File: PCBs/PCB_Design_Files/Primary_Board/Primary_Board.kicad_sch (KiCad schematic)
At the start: 6 parts, among them J1 Conn_FFC_8pin, J2 Conn_01x08_Pin

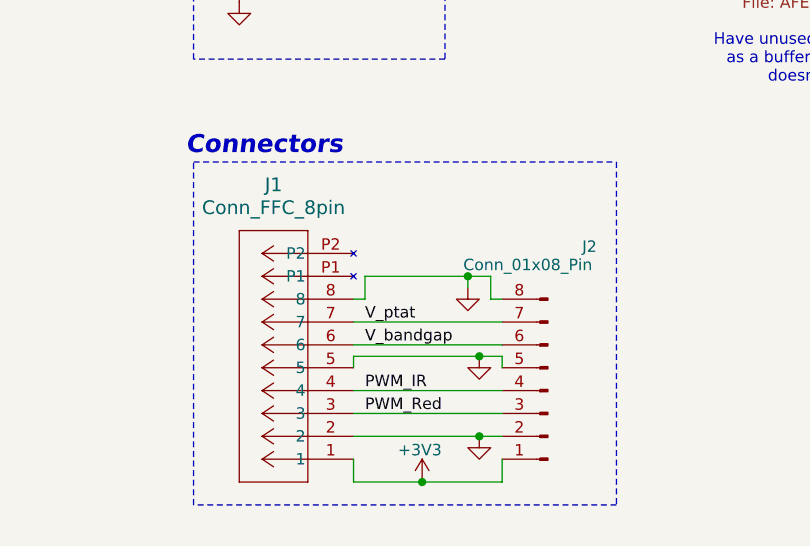
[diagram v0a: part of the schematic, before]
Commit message: updated bom
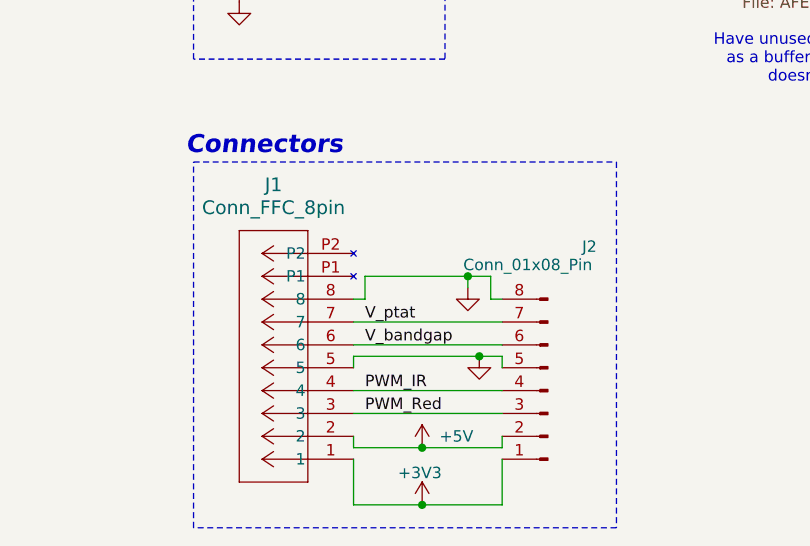
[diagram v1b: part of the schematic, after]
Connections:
- net GND: no longer J1.2, J2.2 (Pin_2)
- new net +5V: J1.2, J2.2 (Pin_2)
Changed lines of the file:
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@@
 	(rectangle
 		(start 25.4 93.98)
-		(end 72.39 132.08)
+		(end 72.39 134.62)
 		(stroke
 			(width 0)
@@
 	)
 	(junction
-		(at 50.8 129.54)
-		(diameter 0)
-		(color 0 0 0 0)
-	)
-	(junction
-		(at 57.15 124.46)
+		(at 50.8 132.08)
 		(diameter 0)
 		(color 0 0 0 0)
@@
 		(color 0 0 0 0)
 	)
+	(junction
+		(at 50.8 125.73)
+		(diameter 0)
+		(color 0 0 0 0)
+	)
 	(wire
 		(pts
@@
 	(wire
 		(pts
+			(xy 59.69 125.73) (xy 59.69 124.46)
+		)
+		(stroke
+			(width 0)
+			(type default)
+		)
+	)
+	(wire
+		(pts
 			(xy 58.42 106.68) (xy 58.42 109.22)
 		)
@@
 	(wire
 		(pts
-			(xy 57.15 124.46) (xy 59.69 124.46)
-		)
-		(stroke
-			(width 0)
-			(type default)
-		)
-	)
-	(wire
-		(pts
 			(xy 43.18 114.3) (xy 59.69 114.3)
 		)
@@
 	(wire
 		(pts
-			(xy 59.69 129.54) (xy 50.8 129.54)
+			(xy 59.69 132.08) (xy 50.8 132.08)
 		)
 		(stroke
@@
 	(wire
 		(pts
+			(xy 43.18 125.73) (xy 43.18 124.46)
+		)
+		(stroke
+			(width 0)
+			(type default)
+		)
+	)
+	(wire
+		(pts
 			(xy 44.45 106.68) (xy 55.88 106.68)
 		)
@@
 	(wire
 		(pts
-			(xy 43.18 127) (xy 43.18 129.54)
+			(xy 43.18 127) (xy 43.18 132.08)
 		)
 		(stroke
@@
 	(wire
 		(pts
-			(xy 43.18 124.46) (xy 57.15 124.46)
+			(xy 43.18 125.73) (xy 50.8 125.73)
 		)
 		(stroke
@@
 	(wire
 		(pts
+			(xy 50.8 125.73) (xy 59.69 125.73)
+		)
+		(stroke
+			(width 0)
+			(type default)
+		)
+	)
+	(wire
+		(pts
 			(xy 43.18 121.92) (xy 59.69 121.92)
 		)
@@
 	(wire
 		(pts
-			(xy 59.69 127) (xy 59.69 129.54)
-		)
-		(stroke
-			(width 0)
-			(type default)
-		)
-	)
-	(wire
-		(pts
-			(xy 43.18 129.54) (xy 50.8 129.54)
+			(xy 59.69 127) (xy 59.69 132.08)
+		)
+		(stroke
+			(width 0)
+			(type default)
+		)
+	)
+	(wire
+		(pts
+			(xy 43.18 132.08) (xy 50.8 132.08)
 		)
 		(stroke
@@
 	(symbol
 		(lib_id "power:+3V3")
-		(at 50.8 129.54 0)
+		(at 50.8 132.08 0)
 		(unit 1)
 		(exclude_from_sim no)
@@
 		(dnp no)
 		(property "Reference" "#PWR023"
-			(at 50.8 133.35 0)
+			(at 50.8 135.89 0)
 			(effects
 				(font
@@
 		)
 		(property "Value" "+3V3"
-			(at 50.546 125.984 0)
+			(at 50.546 128.524 0)
 			(effects
 				(font
@@
 		)
 		(property "Footprint" ""
-			(at 50.8 129.54 0)
+			(at 50.8 132.08 0)
 			(effects
 				(font
@@
 		)
 		(property "Datasheet" ""
-			(at 50.8 129.54 0)
+			(at 50.8 132.08 0)
 			(effects
 				(font
@@
 		)
 		(property "Description" "Power symbol creates a global label with name \"+3V3\""
-			(at 50.8 129.54 0)
+			(at 50.8 132.08 0)
 			(effects
 				(font
@@
 	)
 	(symbol
-		(lib_id "power:GND")
-		(at 57.15 124.46 0)
+		(lib_id "power:VCC")
+		(at 50.8 125.73 0)
 		(unit 1)
 		(exclude_from_sim no)
@@
 		(on_board yes)
 		(dnp no)
-		(fields_autoplaced yes)
 		(property "Reference" "#PWR026"
-			(at 57.15 130.81 0)
-			(effects
-				(font
-					(size 1.27 1.27)
-				)
-				(hide yes)
-			)
-		)
-		(property "Value" "GND"
-			(at 57.1501 128.27 90)
-			(effects
-				(font
-					(size 1.27 1.27)
-				)
-				(justify right)
-				(hide yes)
+			(at 50.8 129.54 0)
+			(effects
+				(font
+					(size 1.27 1.27)
+				)
+				(hide yes)
+			)
+		)
+		(property "Value" "+5V"
+			(at 54.61 124.46 0)
+			(effects
+				(font
+					(size 1.27 1.27)
+				)
 			)
 		)
 		(property "Footprint" ""
-			(at 57.15 124.46 0)
+			(at 50.8 125.73 0)
 			(effects
 				(font
@@
 		)
 		(property "Datasheet" ""
-			(at 57.15 124.46 0)
-			(effects
-				(font
-					(size 1.27 1.27)
-				)
-				(hide yes)
-			)
-		)
-		(property "Description" "Power symbol creates a global label with name \"GND\" , ground"
-			(at 57.15 124.46 0)
-			(effects
-				(font
+			(at 50.8 125.73 0)
+			(effects
+				(font
+					(size 1.27 1.27)
+				)
+				(hide yes)
+			)
+		)
+		(property "Description" "Power symbol creates a global label with name \"VCC\""
+			(at 50.8 125.73 0)
+			(effects
+				(font
